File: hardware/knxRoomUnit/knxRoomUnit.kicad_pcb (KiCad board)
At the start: 2 copper layers, 65 x 42 mm, 69 parts, among them J1 PROG, J2 KNX, P1 ePaper FL, P2 ePaper, Q1 S8050, Q2 S8050, Q3 SI1308, SW1 RESET, SW2 KNX, SW3 DW, SW4 OK, SW5 UP, U1 ESP32-WROOM-32, U2 SHT31-DIS, U3 VCNL4040M3OE

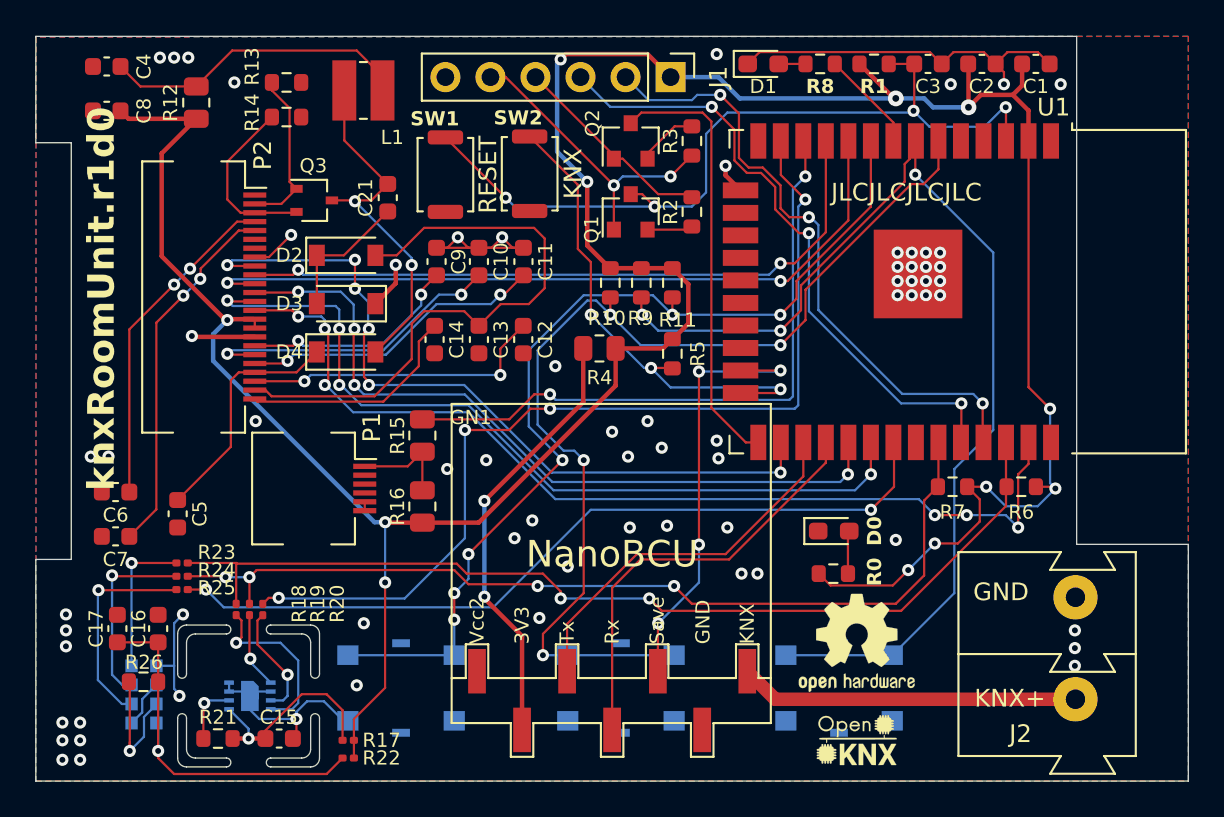
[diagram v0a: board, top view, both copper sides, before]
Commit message: Fixed HW production files
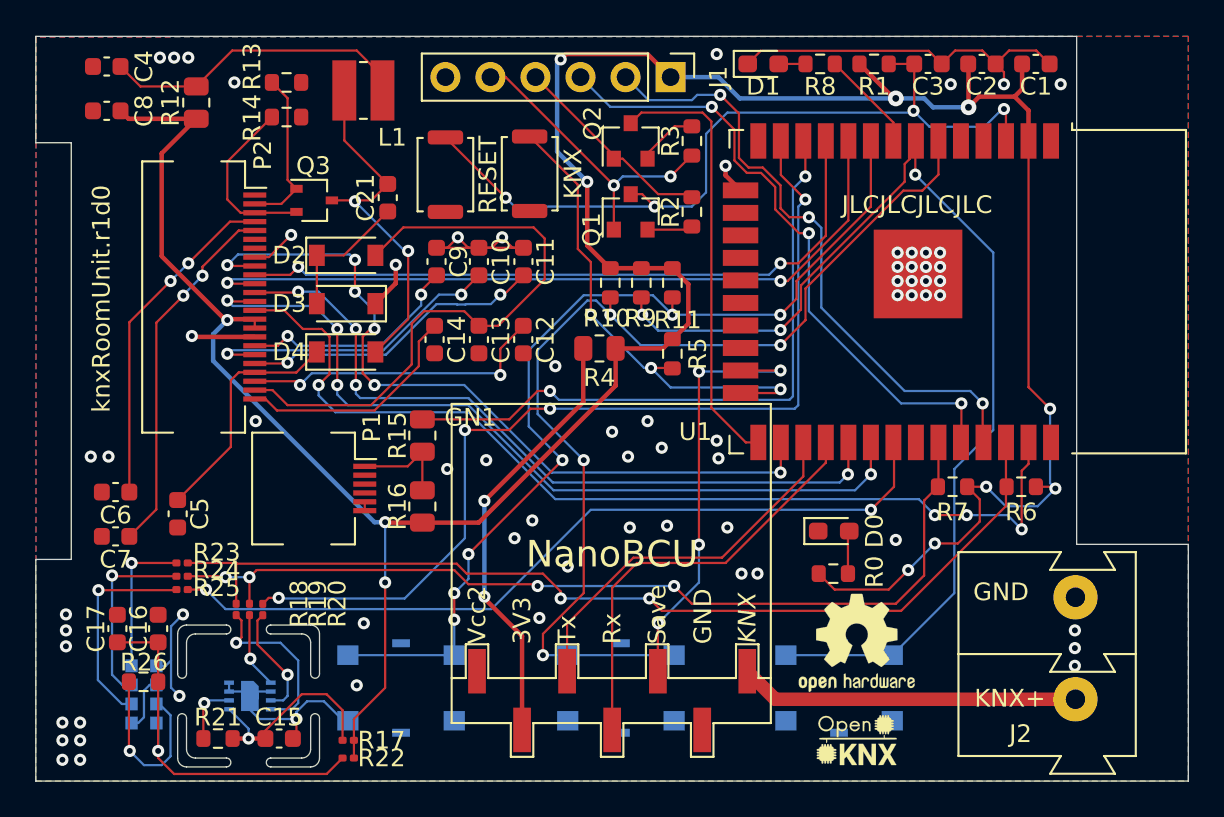
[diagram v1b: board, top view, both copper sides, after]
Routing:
- net Net-(R26-Pad2): track 7.69 -> 10.2 mm
- net EPAPER_BUSY: track 43.4 -> 44.2 mm
- net EPAPER_SDI: track 55.7 -> 56.2 mm, vias 6 -> 4
